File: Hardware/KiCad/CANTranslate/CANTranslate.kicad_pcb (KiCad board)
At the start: 4 copper layers, 51 x 33 mm, 43 parts, among them J1 USB_C_Receptacle_USB2.0_16P, J2 Conn_01x05_Pin, J3 SM04B-GHS-TB(LF)(SN), J4 SM04B-GHS-TB(LF)(SN), SW1 SW_Push, SW2 SW_SPDT, SW3 SW_SPST, U1 USBLC6-2SC6, U2 STM32F303CCT6, U3 AMS1117-3.3, U4 TPS2116DRL, U5 SN65HVD230, Y1 16MHz

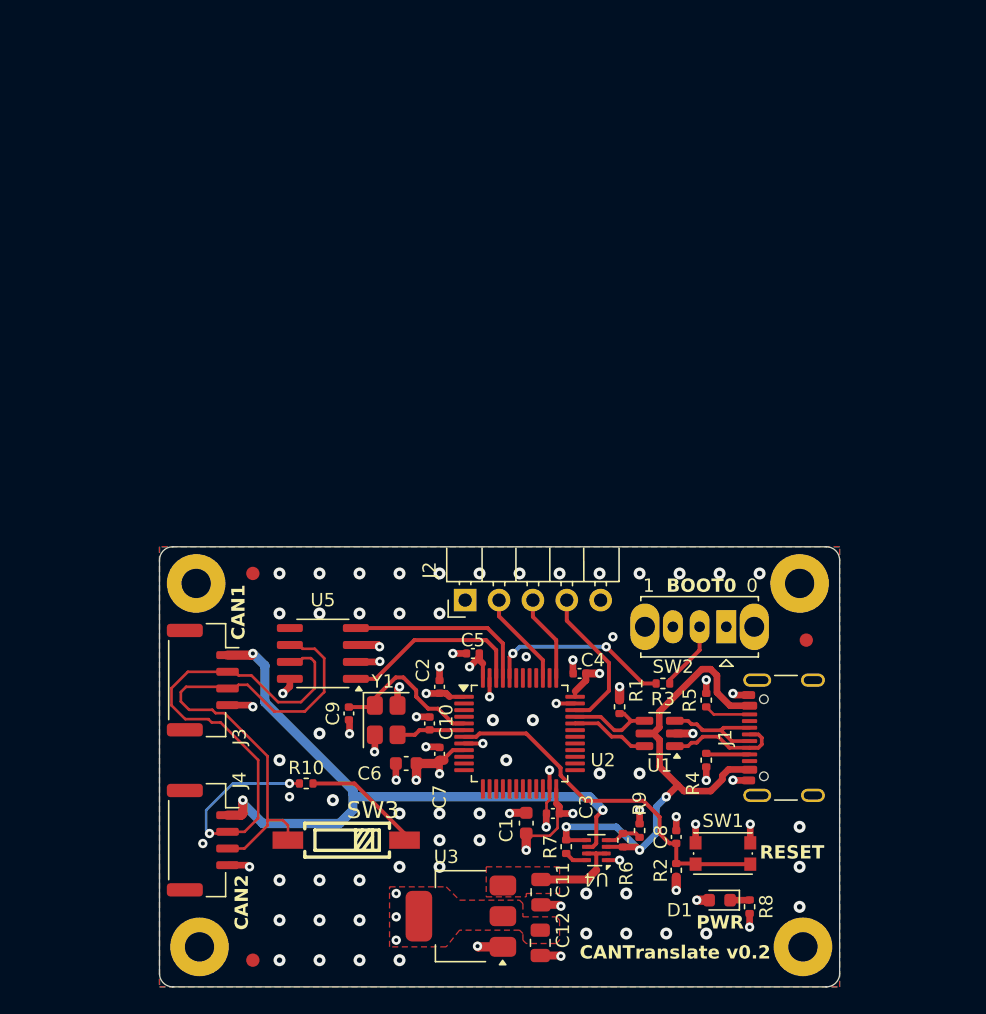
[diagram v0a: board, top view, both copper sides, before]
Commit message: More Hardware Updates
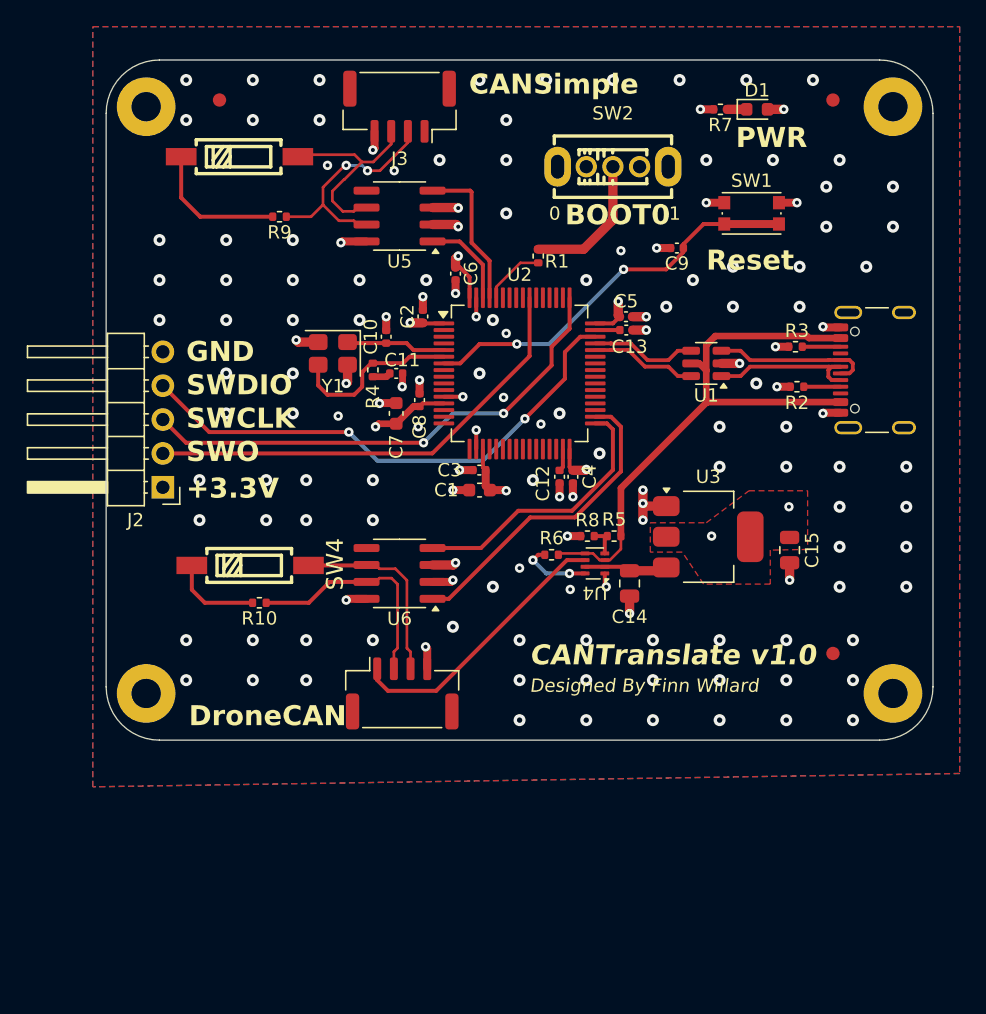
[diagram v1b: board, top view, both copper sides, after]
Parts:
- added C13: 2u2, Capacitor_SMD:C_0402_1005Metric, F.Cu at (215.0, 51.8)
- added C14: 22u, Capacitor_SMD:C_0805_2012Metric, F.Cu at (215.2, 70.8)
- added C15: 22u, Capacitor_SMD:C_0805_2012Metric, F.Cu at (227.2, 68.2)
- added SW4: SW_SPST, DSIC01LSGET:SW-SMD_DSIC01LSGET, F.Cu at (186.8, 69.4)
- added U6: SN65HVD230, Package_SO:SOIC-8_3.9x4.9mm_P1.27mm, F.Cu at (198.0, 70.0)
- C11: value 22u -> 10p; footprint Capacitor_SMD:C_0805_2012Metric -> Capacitor_SMD:C_0402_1005Metric
- C12: value 22u -> 2u2; footprint Capacitor_SMD:C_0805_2012Metric -> Capacitor_SMD:C_0402_1005Metric
- C6: value 1u -> 100n; footprint Capacitor_SMD:C_0603_1608Metric -> Capacitor_SMD:C_0402_1005Metric
- C7: value 100n -> 1u; footprint Capacitor_SMD:C_0402_1005Metric -> Capacitor_SMD:C_0603_1608Metric
- C9: value 10p -> 100n
- R1: value 1k5 -> 10k
- R2, R3: value 10k -> 5k1
- R4: value 5k1 -> 470
- R5: value 5k1 -> 36k
- R6: value 36k -> 10k
- R7, R9: value 10k -> 120
- R8: value 120 -> 10k
- SW2: footprint Button_Switch_THT:SW_Slide_SPDT_Straight_CK_OS102011MS2Q -> easyeda2kicad:SW-TH_SS12D07VG4
- U2: value STM32F303CCT6 -> STM32F205RGT6; footprint Package_QFP:LQFP-48_7x7mm_P0.5mm -> Package_QFP:LQFP-64_10x10mm_P0.5mm
- moved H2 63.3 mm to (235.0, 35.0)
- moved H1 60.7 mm to (179.0, 35.0)
- moved D1 59.4 mm to (224.8, 35.2), turned to 0 degrees
- moved R7 56.5 mm to (222.1, 35.2), turned to 180 degrees
- moved H4 55.4 mm to (235.0, 79.0)
- moved R9 53.4 mm to (189.0, 43.2), turned to 180 degrees
- moved H3 52.8 mm to (179.0, 79.0)
- moved SW3 51.9 mm to (186.0, 38.8), turned to -90 degrees
- moved FID3 49.2 mm to (230.5, 76.0)
- moved SW1 48.0 mm to (224.4, 43.0)
- moved J3 45.5 mm to (198.0, 35.0), turned to 180 degrees
- moved C9 42.7 mm to (218.8, 45.6), turned to 180 degrees
- moved FID2 40.5 mm to (230.5, 34.5)
- moved C11 40.4 mm to (197.8, 55.0), turned to 0 degrees
- moved R4 38.5 mm to (196.0, 54.7)
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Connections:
- C10 pad 1: /HSE_OUT -> /HSE_IN
- C11 pad 1: /V_OUT -> Net-(C11-Pad1)
- C12 pad 1: +3.3V -> /VCAP_1
- C8 pad 1: /NRST -> +3.3V
- C9 pad 1: /HSE_IN -> /NRST
- J3 pad 1: +5V -> unconnected-(J3-Pad1)
- J3 pad 2: /CAN+ -> /CAN1+
- J3 pad 3: /CAN- -> /CAN1-
- J4 pad 2: /CAN+ -> /CAN2+
- J4 pad 3: /CAN- -> /CAN2-
- R1 pad 1: +3.3V -> /S_BOOT0
- R1 pad 2: /USB_D+ -> /BOOT0
- R10 pad 1: /CAN+ -> /CAN2+
- R10 pad 2: Net-(SW3-B) -> Net-(SW4-B)
- R2 pad 1: +3.3V -> /USBCC1
- R2 pad 2: /NRST -> GND
- R3 pad 1: /S_BOOT0 -> /USBCC2
- R3 pad 2: /BOOT0 -> GND
- R4 pad 1: /USBCC1 -> /HSE_OUT
- R4 pad 2: GND -> Net-(C11-Pad1)
- R5 pad 1: /USBCC2 -> VBUS
- R5 pad 2: GND -> /V_PR1
- R6 pad 2: /V_PR1 -> Net-(U4-ST)
- R7 pad 1: VBUS -> Net-(D1-K)
- R7 pad 2: Net-(U4-ST) -> GND
- R8 pad 1: Net-(D1-K) -> /V_PR1
- R9 pad 1: /V_PR1 -> /CAN1+
- R9 pad 2: GND -> Net-(SW3-B)
- SW3 pad 1: /CAN- -> /CAN1-
- U2 pad 12: unconnected-(U2-PA2-Pad12) -> GND
- U2 pad 13: unconnected-(U2-PA3-Pad13) -> +3.3V
- U2 pad 18: unconnected-(U2-PB0-Pad18) -> GND
- U2 pad 19: unconnected-(U2-PB1-Pad19) -> +3.3V
- U2 pad 23: GND -> unconnected-(U2-PA7-Pad23)
- U2 pad 24: +3.3V -> unconnected-(U2-PC4-Pad24)
- U2 pad 31: unconnected-(U2-PA10-Pad31) -> /VCAP_1
- U2 pad 32: /USB_D- -> +3.3V
- U2 pad 33: /USB_D+ -> /CAN2_RX
- U2 pad 34: /SWDIO -> /CAN2_TX
- U2 pad 35: GND -> unconnected-(U2-PB14-Pad35)
- U2 pad 36: +3.3V -> unconnected-(U2-PB15-Pad36)
- U2 pad 37: /SWCLK -> unconnected-(U2-PC6-Pad37)
- U2 pad 39: /SWO -> unconnected-(U2-PC8-Pad39)
- U2 pad 44: /BOOT0 -> /USB_D-
- U2 pad 45: /CAN_RX -> /USB_D+
- U2 pad 46: /CAN_TX -> /SWDIO
- U2 pad 47: GND -> /VCAP_2
- U2 pad 8: GND -> unconnected-(U2-PC0-Pad8)
- U2 pad 9: +3.3V -> unconnected-(U2-PC1-Pad9)
- U5 pad 1: /CAN_TX -> /CAN1_TX
- U5 pad 4: /CAN_RX -> /CAN1_RX
- U5 pad 6: /CAN- -> /CAN1-
- U5 pad 7: /CAN+ -> /CAN1+
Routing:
- net /CAN+: track 44.4 -> 0.00 mm, vias 2 -> 0
- net /CAN-: track 38.7 -> 0.00 mm
- net /SWCLK: track 6.56 -> 37.9 mm, vias 0 -> 2
- net +5V: track 51.4 -> 20.8 mm, vias 3 -> 0
- net /SWDIO: track 11.2 -> 39.8 mm, vias 0 -> 2
- net /SWO: track 7.20 -> 34.9 mm
- net /CAN2_TX: track 0.00 -> 23.7 mm
- net /CAN2_RX: track 0.00 -> 20.5 mm
- net /CAN2+: track 0.00 -> 17.3 mm
- net /CAN1+: track 0.00 -> 17.2 mm, vias 0 -> 2
- net /CAN1-: track 0.00 -> 15.6 mm
- net /CAN2-: track 0.00 -> 14.6 mm
- net /CAN_TX: track 14.1 -> 0.00 mm
- net /CAN_RX: track 14.1 -> 0.00 mm
- net /CAN1_RX: track 0.00 -> 11.5 mm
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- removed copper zone on F.Cu, net /V_OUT
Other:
- board size 51 x 33 mm -> 62 x 51 mm
- board text added: "+3.3V"
- board text added: "CANSimple"
- board text added: "CANTranslate v1.0"
- board text added: "Designed By Finn Willard"
- board text added: "DroneCAN"
- board text added: "Reset"
- board text removed: "3.3V"
- board text removed: "CAN1"
- board text removed: "CAN2"
- board text removed: "CANTranslate v0.2"
- board text removed: "RESET"
